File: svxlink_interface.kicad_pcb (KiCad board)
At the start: 2 copper layers, 20 parts, among them J1 MTM5400 acc.con., J2 RCJ-2123, J3 RPi-GPIO xx, J5 FTDI USB>UART, T1-RX1 600ohm 1:1, T2-TX1 600ohm 1:1, U1 CNY17-2

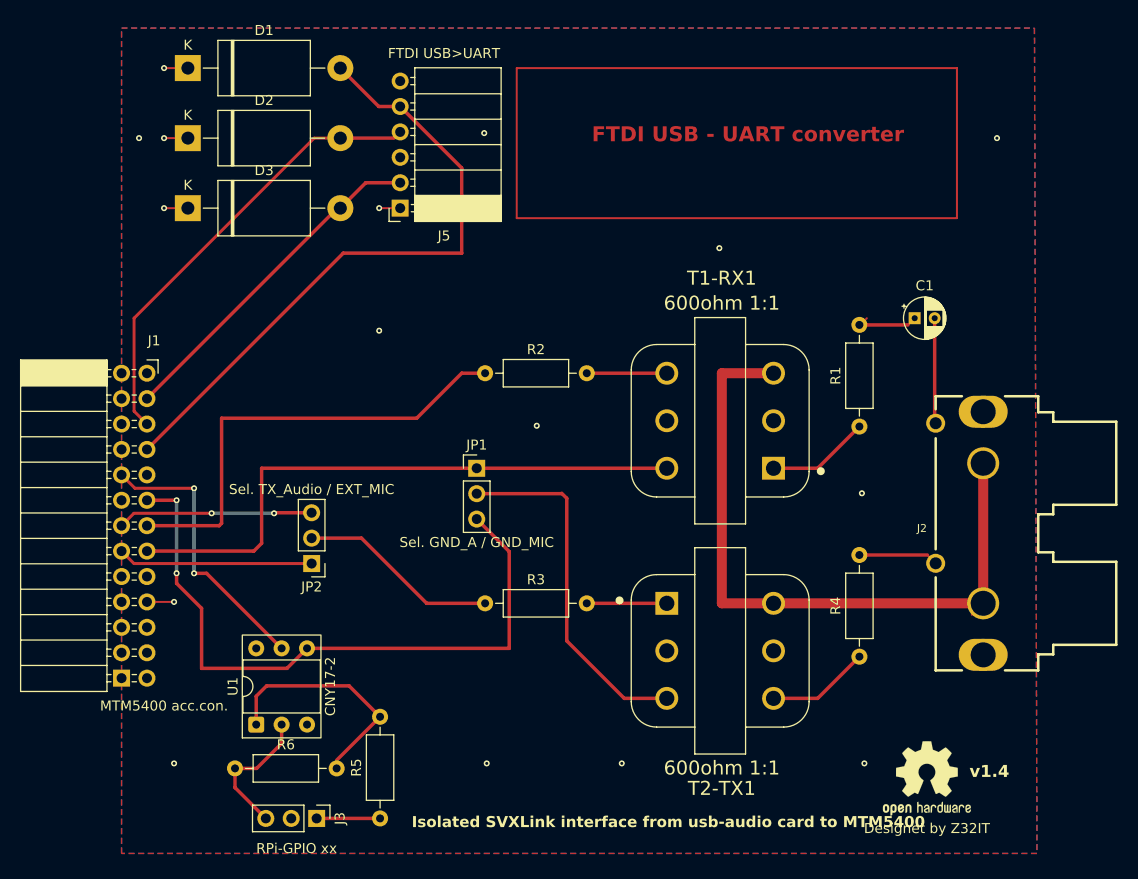
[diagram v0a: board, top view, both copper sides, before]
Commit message: Add files via upload
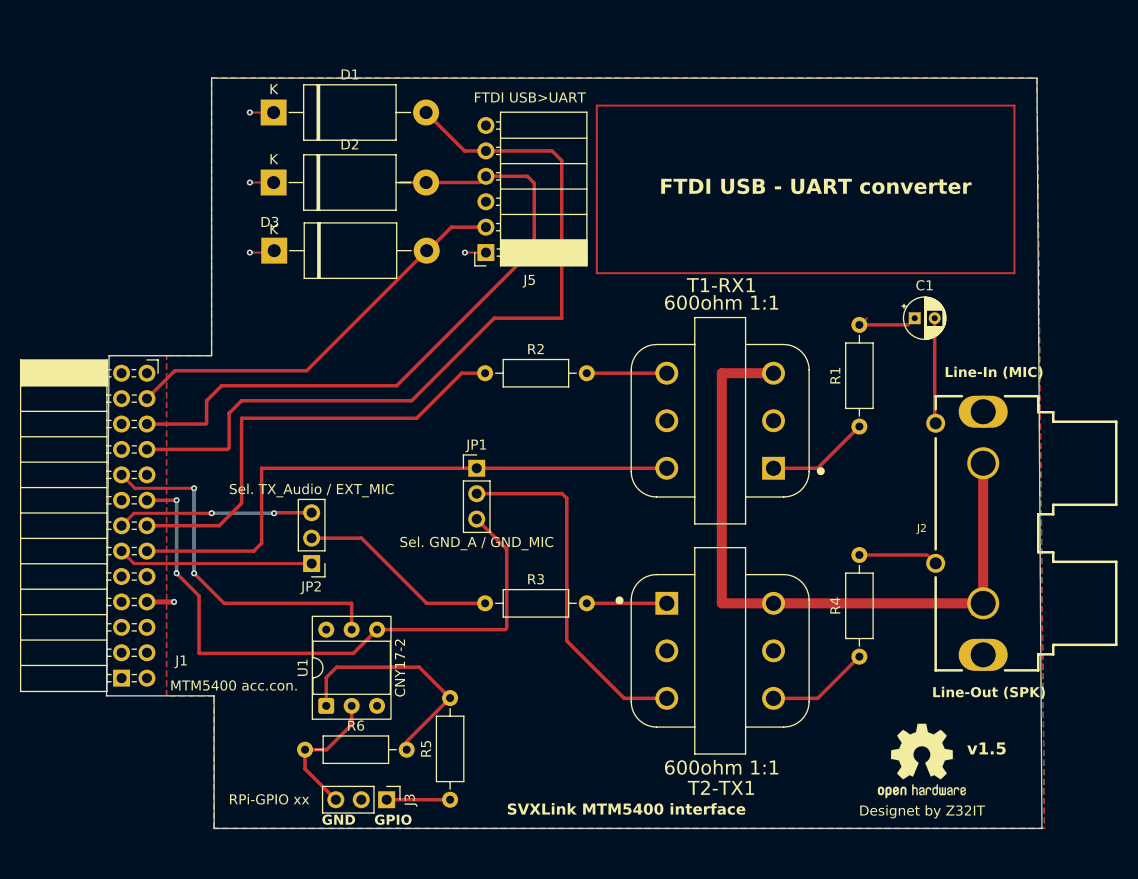
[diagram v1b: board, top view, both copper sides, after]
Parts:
- moved J5 9.65 mm to (84.9, 52.4)
- moved D1 9.65 mm to (63.7, 38.4)
- moved D2 9.65 mm to (63.7, 45.4)
- moved D3 9.62 mm to (63.8, 52.2)
- moved J3 7.25 mm to (75.0, 107.1)
- moved R5 7.25 mm to (81.3, 107.1)
- moved R6 7.25 mm to (66.8, 102.1)
- moved U1 7.25 mm to (69.0, 97.8)
- moved REF** 1.82 mm to (128.5, 103.2)
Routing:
- net TXD: track 45.4 -> 67.8 mm
- net RXD: track 64.4 -> 80.3 mm
- net Net-(J1-PTT): track 28.2 -> 35.9 mm
- net CTS: track 34.2 -> 41.4 mm
- net GND_MIC: track 66.6 -> 63.1 mm
- net Net-(J1-RX_Audio): track 46.3 -> 45.1 mm
- net GND: vias 16 -> 5
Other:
- board outline added: 93.5 x 75 mm
- board text added: "${REFERENCE}"
- board text added: "GND"
- board text added: "GPIO"
- board text added: "K"
- board text added: "Line-In (MIC)"
- board text added: "Line-Out (SPK)"
- board text added: "SVXLink MTM5400 interface"
- board text added: "v1.5"
- board text removed: "Isolated SVXLink interface from usb-audio card to MTM5400"
- board text removed: "v1.4"
